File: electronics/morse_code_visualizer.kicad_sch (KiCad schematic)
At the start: 12 parts, among them SW1 Push_Button

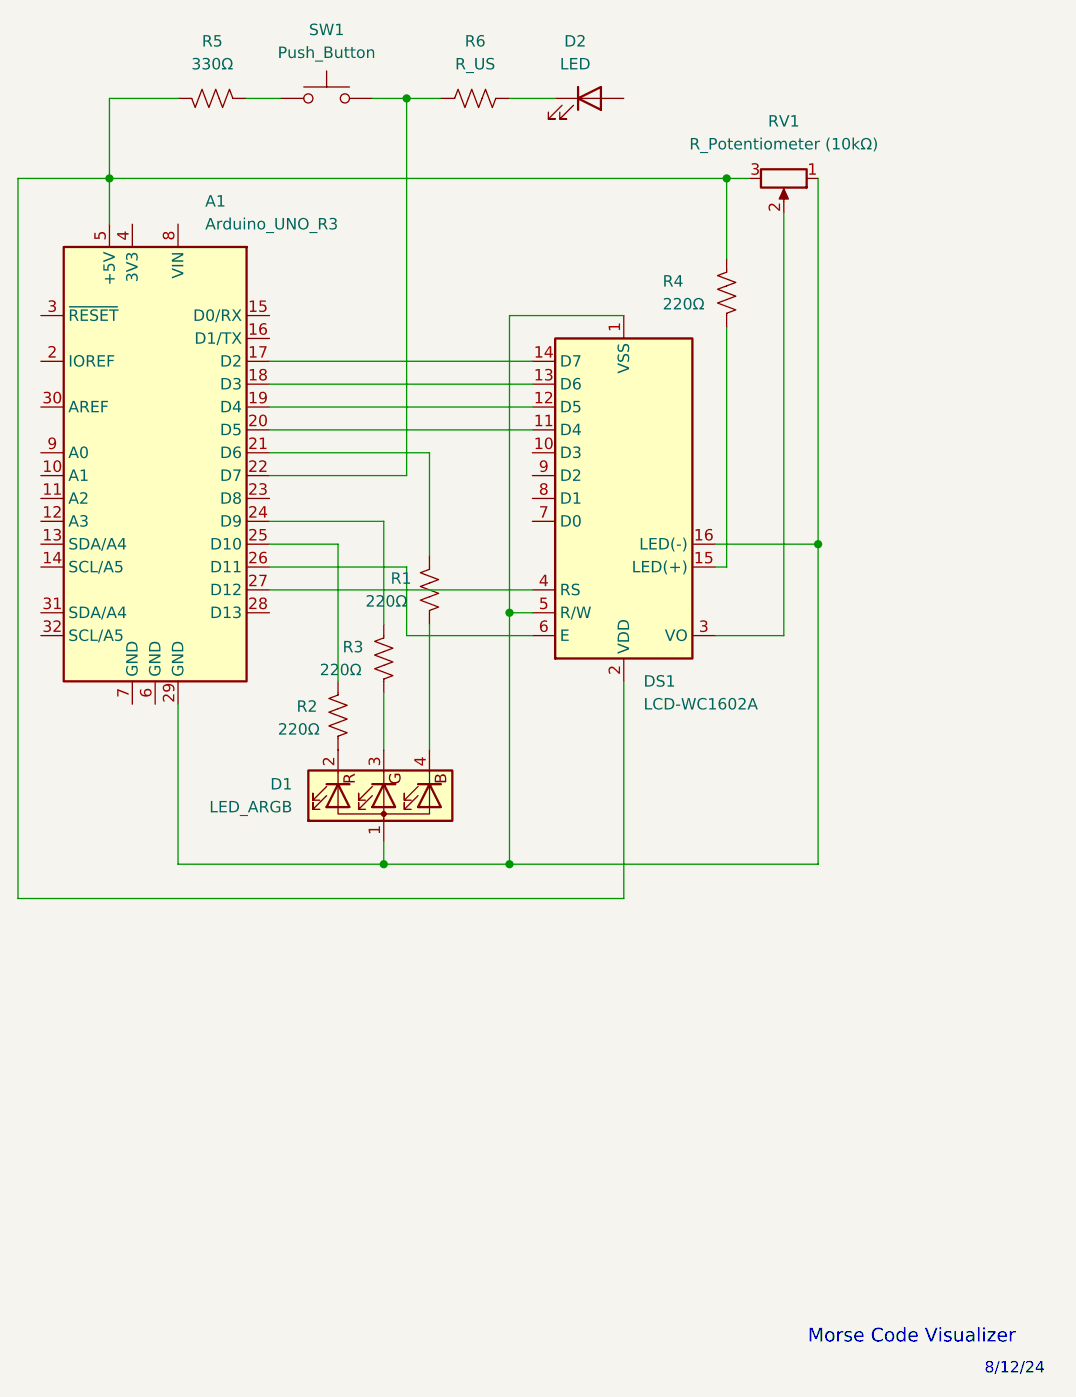
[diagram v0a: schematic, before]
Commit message: Updated schematic
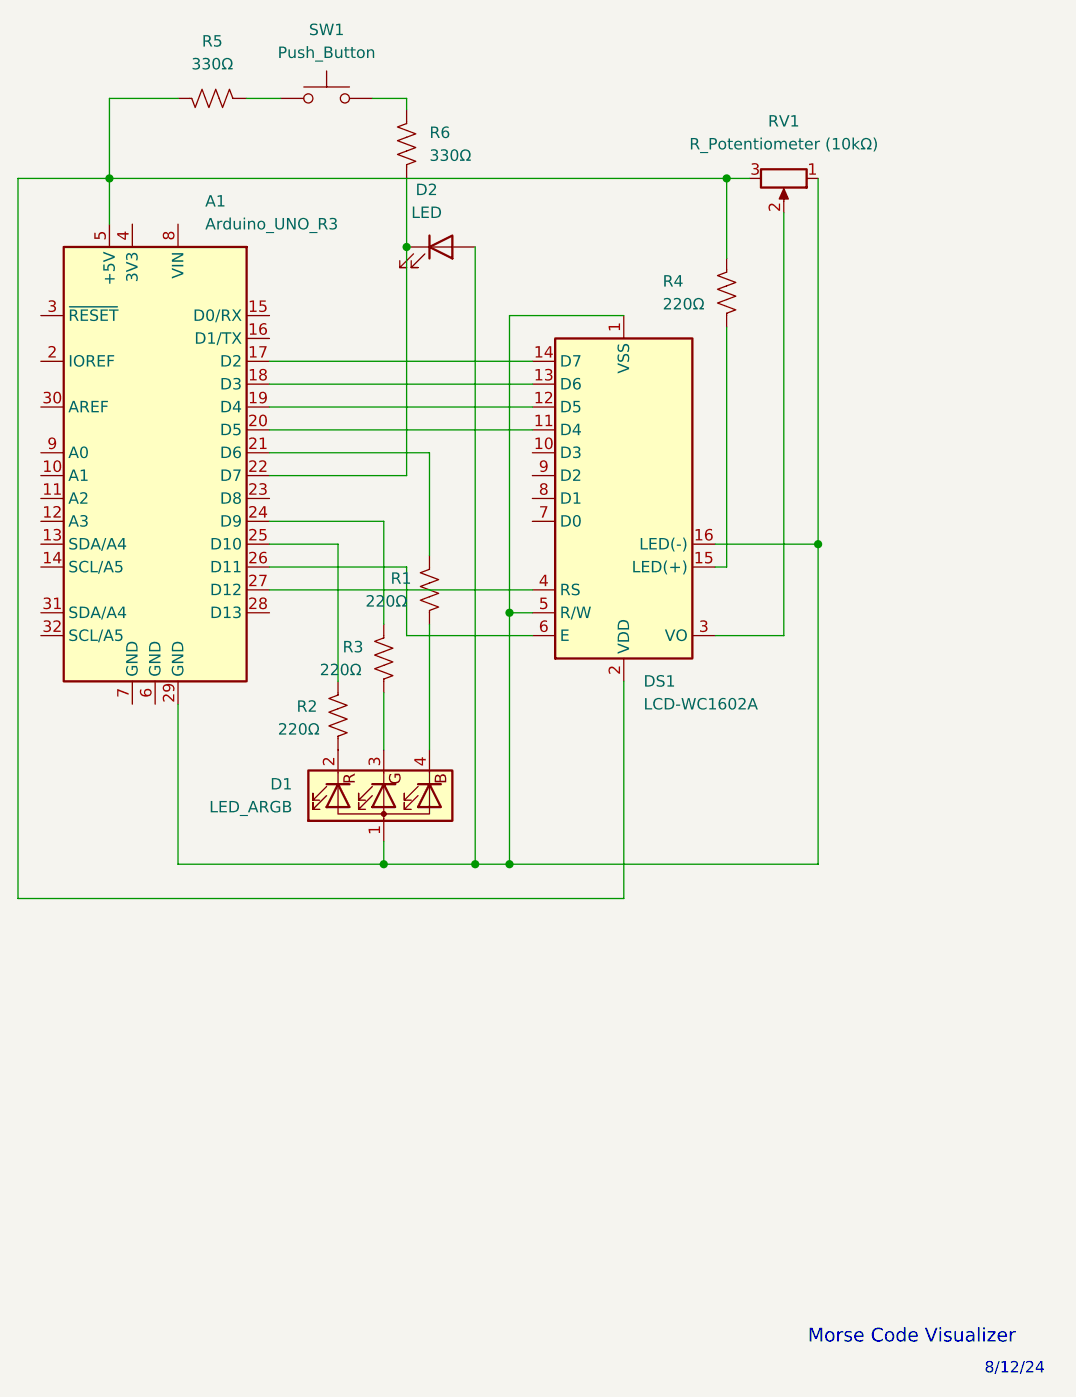
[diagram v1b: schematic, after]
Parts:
- R6: value R_US -> 330Ω
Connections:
- net at D2.1 (K), R6.2: now also A1.22 (D7)
- net at D2.2 (A): now also A1.29 (GND), D1.1 (A), DS1.1 (VSS), DS1.16 (LED(-)), DS1.5 (R/W), RV1.1
- net at R6.1, SW1.1: no longer A1.22 (D7)
